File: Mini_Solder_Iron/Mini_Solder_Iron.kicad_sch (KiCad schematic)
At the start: 9 parts, among them CN1 YXT-BB10-24S-02, J1 USB_C_Receptacle_USB2.0, Q1 AO4407A, U1 STM32F103C8Tx, U2 LIS2DS12, U3 SGM8557, U4 TMP36GRTZ, U5 CH224K, U6 MP9942

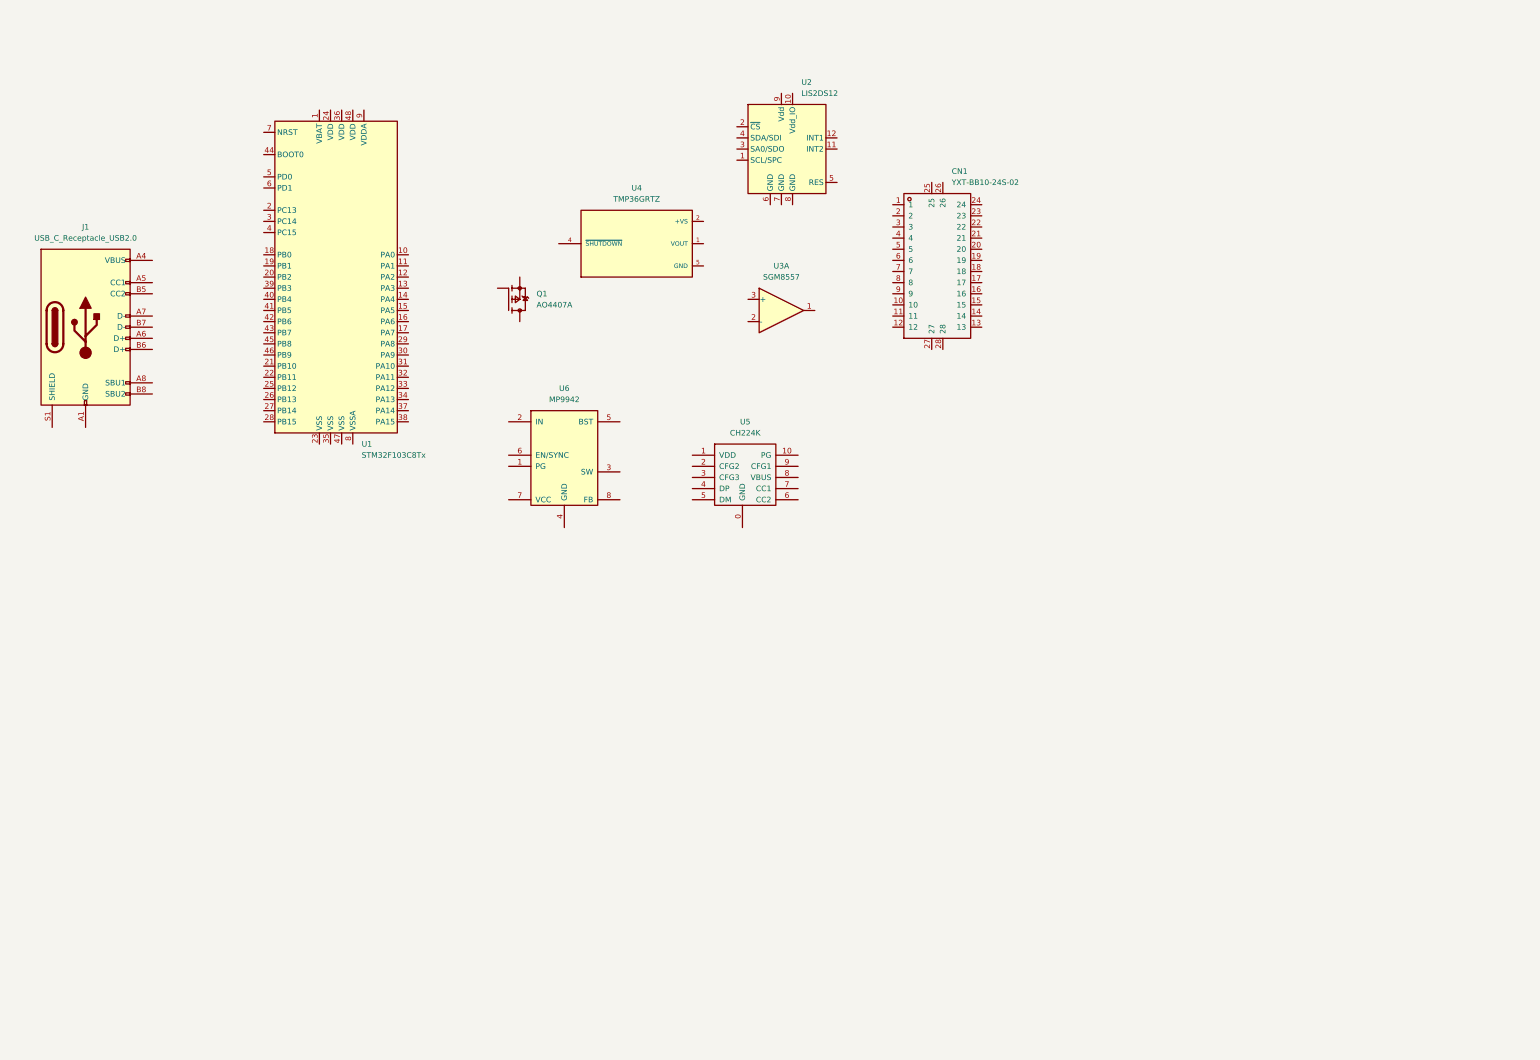
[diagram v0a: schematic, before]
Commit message: update
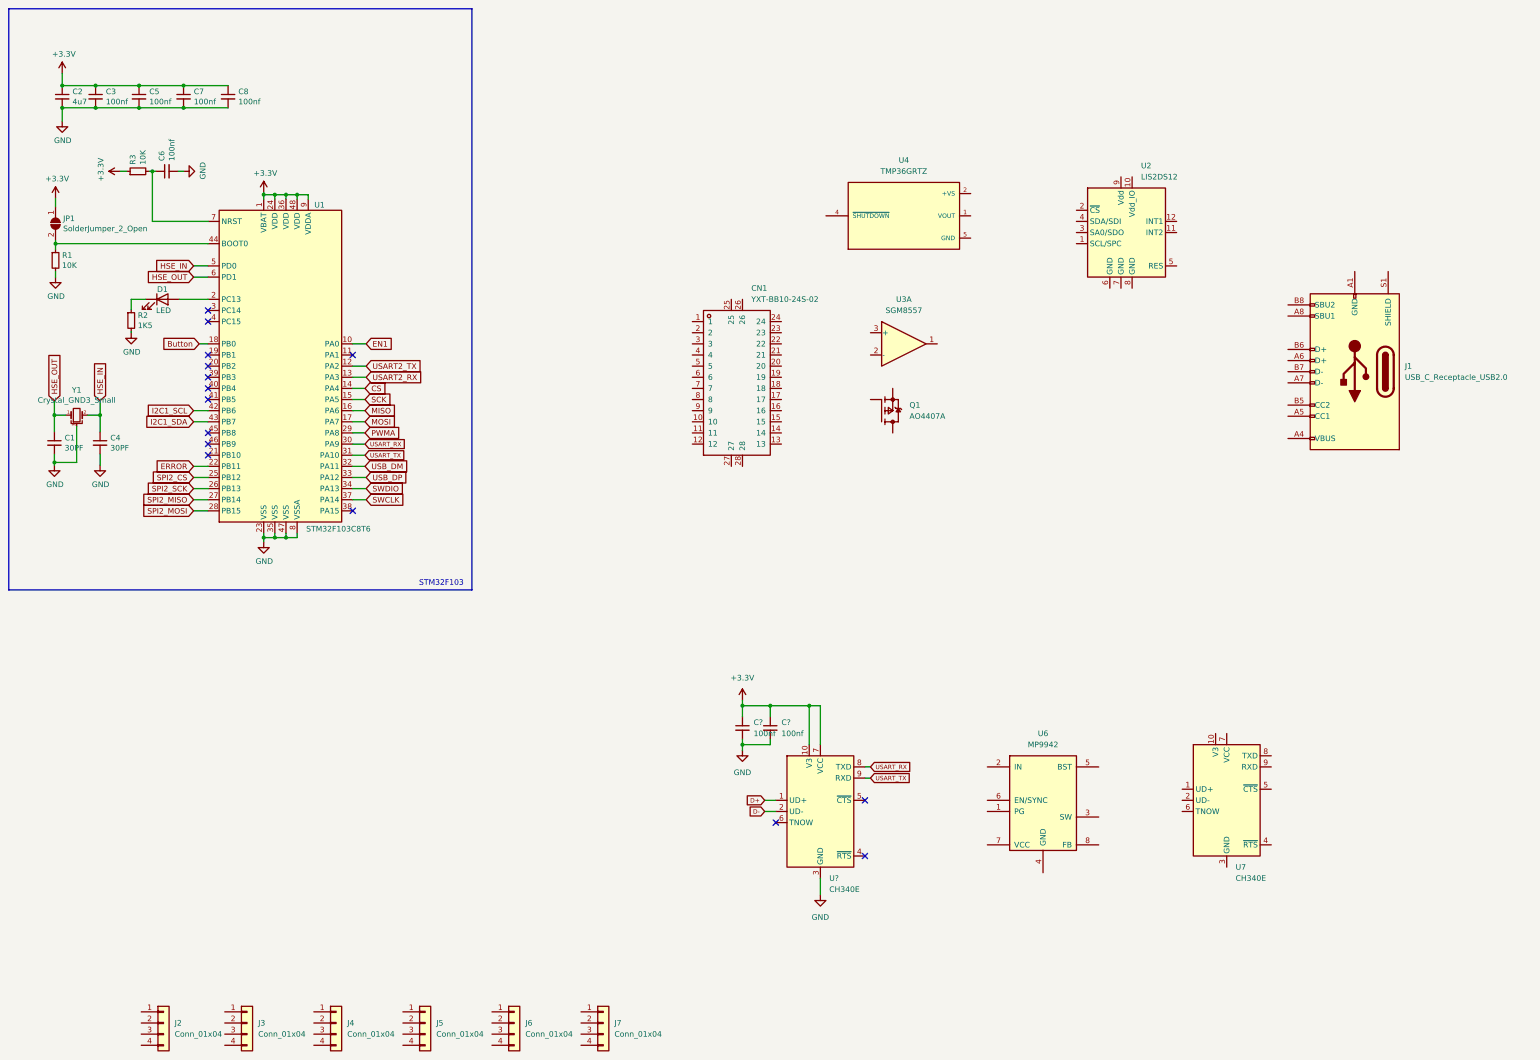
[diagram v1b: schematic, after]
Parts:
- removed U5: CH224K, kicad_lceda:ESSOP-10_L4.9-W3.9-P1.0-LS6.0-TL-EP, symbol kicad_lceda:CH224K
- added C1, C4: 30PF, Capacitor_SMD:C_0402_1005Metric, symbol Device:C_Small
- added C2: 4u7, Capacitor_SMD:C_0402_1005Metric, symbol Device:C_Small
- added C3, C5, C6, C7, C8: 100nf, Capacitor_SMD:C_0402_1005Metric, symbol Device:C_Small
- added C? (x2): 100nf, Capacitor_SMD:C_0402_1005Metric_Pad0.74x0.62mm_HandSolder, symbol Device:C_Small
- added D1: LED, LED_SMD:LED_0402_1005Metric, symbol Device:LED
- added J2, J5: Conn_01x04, kicad_lceda:JBC245_2.4mm, symbol Connector_Generic:Conn_01x04
- added J3, J6: Conn_01x04, kicad_lceda:JBC245_1.5mm, symbol Connector_Generic:Conn_01x04
- added J4, J7: Conn_01x04, kicad_lceda:JBC245_3.5mm, symbol Connector_Generic:Conn_01x04
- added JP1: SolderJumper_2_Open, Jumper:SolderJumper-2_P1.3mm_Open_RoundedPad1.0x1.5mm, symbol Jumper:SolderJumper_2_Open
- added R1, R3: 10K, Resistor_SMD:R_0402_1005Metric, symbol Device:R_Small
- added R2: 1K5, Resistor_SMD:R_0402_1005Metric, symbol Device:R_Small
- added U7, U?: CH340E, Package_SO:MSOP-10_3x3mm_P0.5mm, symbol Interface_USB:CH340E
- added Y1: Crystal_GND3_Small, CSTCE8M00G55:OSC_CSTCE8M00G55-R0, symbol Device:Crystal_GND3_Small
- U1: value STM32F103C8Tx -> STM32F103C8T6
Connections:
- net +3V3: now reaches U1.1 (VBAT)
- net +3V3: now also U1.24 (VDD), U1.36 (VDD), U1.48 (VDD), U1.9 (VDDA), C2.1, C3.1, C5.1, C7.1, C8.1, C?.1, C?.1, JP1.1 (A), R3.1, U?.10 (V3), U?.7 (VCC)
- net EN1: now reaches U1.10 (PA0)
- net USART2_TX: now reaches U1.12 (PA2)
- net USART2_RX: now reaches U1.13 (PA3)
- net CS: now reaches U1.14 (PA4)
- net SCK: now reaches U1.15 (PA5)
- net MISO: now reaches U1.16 (PA6)
- net MOSI: now reaches U1.17 (PA7)
- net Button: now reaches U1.18 (PB0)
- net at U1.2 (PC13): now also D1.2 (A)
- net ERROR: now reaches U1.22 (PB11)
- net GND: now reaches U1.23 (VSS)
- net GND: now also U1.35 (VSS), U1.47 (VSS), U1.8 (VSSA), C1.2, C2.2, C3.2, C4.2, C5.2, C6.2, C7.2, C8.2, C?.2, C?.2, R1.2, R2.2, U?.3 (GND), Y1.3
- net SPI2_CS: now reaches U1.25 (PB12)
- net SPI2_SCK: now reaches U1.26 (PB13)
- net SPI2_MISO: now reaches U1.27 (PB14)
- net SPI2_MOSI: now reaches U1.28 (PB15)
- net PWMA: now reaches U1.29 (PA8)
- net USART_RX: now reaches U1.30 (PA9)
- net USART_RX: now also U?.8 (TXD)
- net USART_TX: now reaches U1.31 (PA10)
- net USART_TX: now also U?.9 (RXD)
- net USB_DM: now reaches U1.32 (PA11)
- net USB_DP: now reaches U1.33 (PA12)
- net SWDIO: now reaches U1.34 (PA13)
- net SWCLK: now reaches U1.37 (PA14)
- net I2C1_SCL: now reaches U1.42 (PB6)
- net I2C1_SDA: now reaches U1.43 (PB7)
- net at U1.44 (BOOT0): now also JP1.2 (B), R1.1
- net HSE_IN: now reaches U1.5 (PD0)
- net HSE_IN: now also C4.1, Y1.2
- net HSE_OUT: now reaches U1.6 (PD1)
- net HSE_OUT: now also C1.1, Y1.1
- net at U1.7 (NRST): now also C6.1, R3.2
- new net: D1.1 (K), R2.1
- new net D+: U?.1 (UD+)
- new net D-: U?.2 (UD-)
- no-connect marks 0 -> 15
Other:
- note added: "STM32F103"
- moved on the sheet: CN1, J1, Q1, U2, U3A, U4, U6
